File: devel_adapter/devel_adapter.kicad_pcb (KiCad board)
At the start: 4 copper layers, 49.5 x 15.2 mm, 4 parts, among them J1 Conn_02x20_Odd_Even, J2 Conn_01x20, J3 Conn_01x20

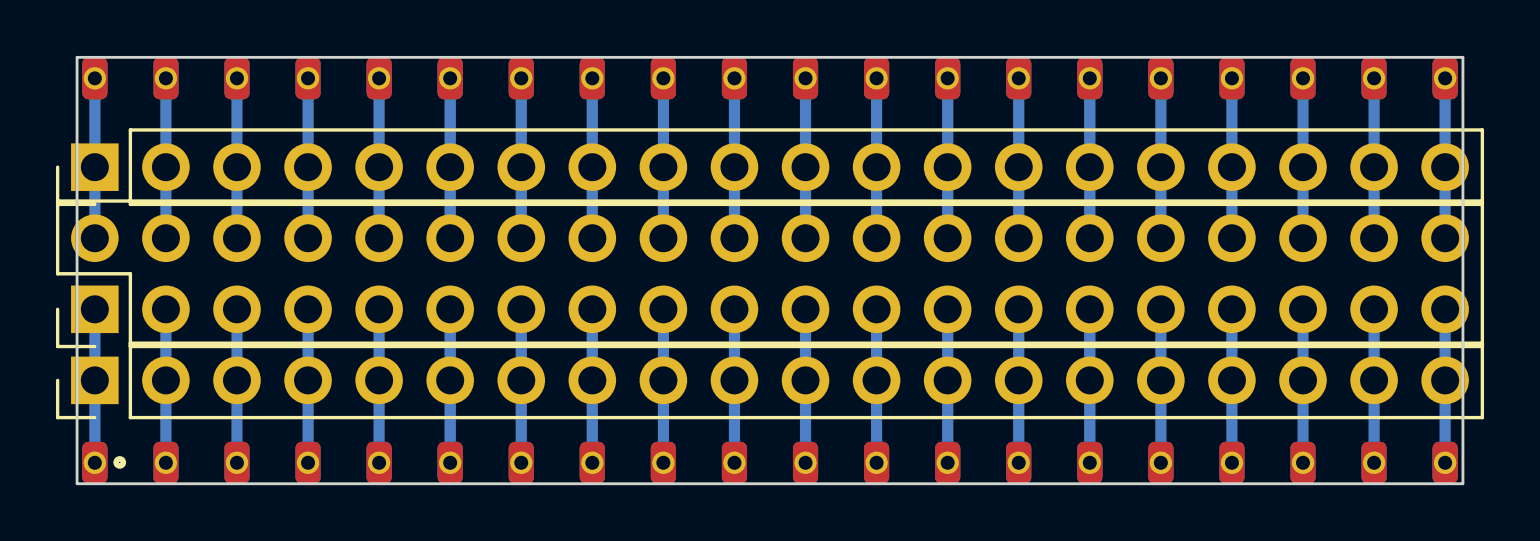
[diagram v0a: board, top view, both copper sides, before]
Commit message: Adapter board is production ready
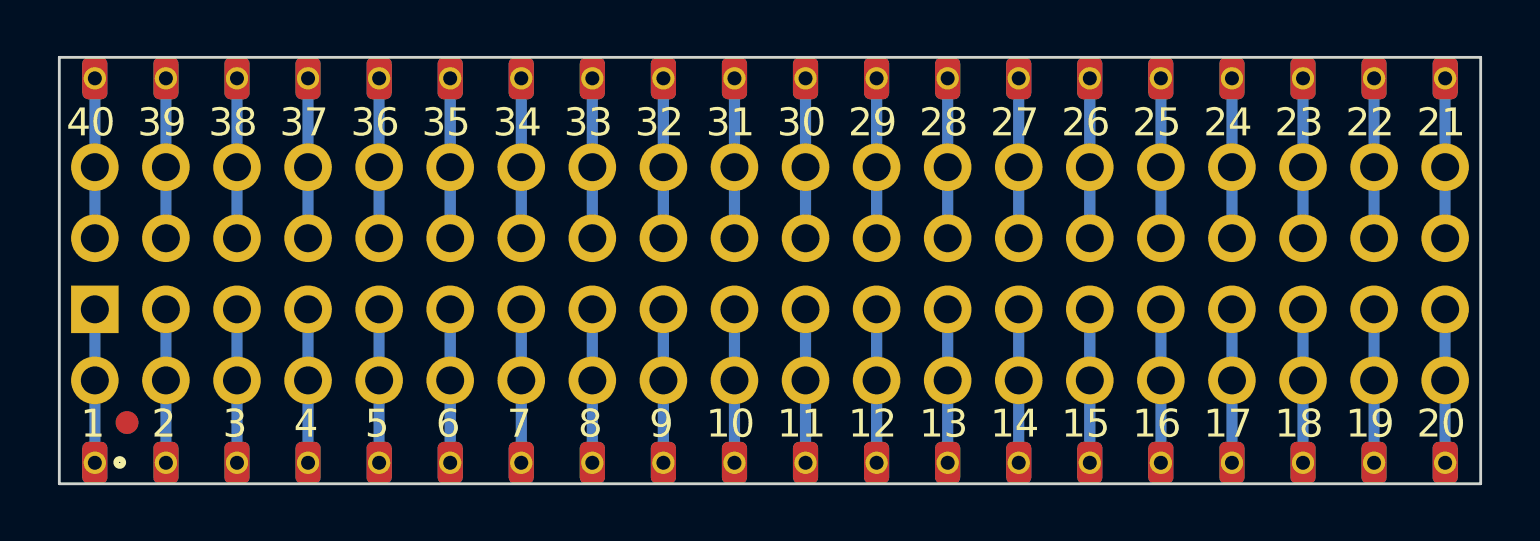
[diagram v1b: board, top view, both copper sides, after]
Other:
- board size 49.5 x 15.2 mm -> 50.8 x 15.2 mm
- copper layers 4 -> 2
- board text added: "1"
- board text added: "10"
- board text added: "11"
- board text added: "12"
- board text added: "13"
- board text added: "14"
- board text added: "15"
- board text added: "16"
- board text added: "17"
- board text added: "18"
- board text added: "19"
- board text added: "2"
- board text added: "20"
- board text added: "21"
- board text added: "22"
- board text added: "23"
- board text added: "24"
- board text added: "25"
- board text added: "26"
- board text added: "27"
- board text added: "28"
- board text added: "29"
- board text added: "3"
- board text added: "30"
- board text added: "31"
- board text added: "32"
- board text added: "33"
- board text added: "34"
- board text added: "35"
- board text added: "36"
- board text added: "37"
- board text added: "38"
- board text added: "39"
- board text added: "4"
- board text added: "40"
- board text added: "5"
- board text added: "6"
- board text added: "7"
- board text added: "8"
- board text added: "9"
